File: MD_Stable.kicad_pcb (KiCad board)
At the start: 2 copper layers, 100 x 100 mm, 308 parts, among them J1 Conn_02x04_Counter_Clockwise, J10 Conn_02x06_Odd_Even, J11 Conn_01x08_Pin, J12 Conn_01x05_Socket, J2 XT30_Male, J3 XT60_Male, J4 RE1, J5 RE2, J6 RE3, J7 MO_XT60_Female1, J8 MO_XT60_Female2, J9 MO_XT60_Female3, Q1 MTB7D0N6RJ3, Q10 MTB7D0N6RJ3, Q11 MTB7D0N6RJ3, Q12 MTB7D0N6RJ3, Q2 MTB7D0N6RJ3, Q3 MTB7D0N6RJ3, Q4 MTB7D0N6RJ3, Q5 MTB7D0N6RJ3, Q6 MTB7D0N6RJ3, Q7 MTB7D0N6RJ3, Q8 MTB7D0N6RJ3, Q9 MTB7D0N6RJ3, SW1 SW_Push, SW2 SW_Push, SW3 PWM, SW4 PWM, SW5 PWM, SW6 DIR, SW7 DIR, SW8 DIR, U1 NJM7808SDL1, U10 74AHC1G08W5, U11 74AHC1G08W5, U12 74AHC1G08W5, U13 IRS2302S, U14 IRS2302S, U15 IRS2302S, U16 NE555D, U17 IRS2302S, U18 IRS2302S, U19 IRS2302S, U2 BA05CC0Tに似た何か, U20 74AHC1G08W5, U21 74AHC1G08W5, U22 74AHC1G08W5, U23 UTRS485G-S08-R, U24 UTRS485G-S08-R, U3 STM32G431K8Tx, U4 BA05CC0Tに似た何か, U5 BA033CC0FP, U6 π160M60, U7 74AHC1G04W5, U8 74AHC1G04W5, U9 74AHC1G04W5

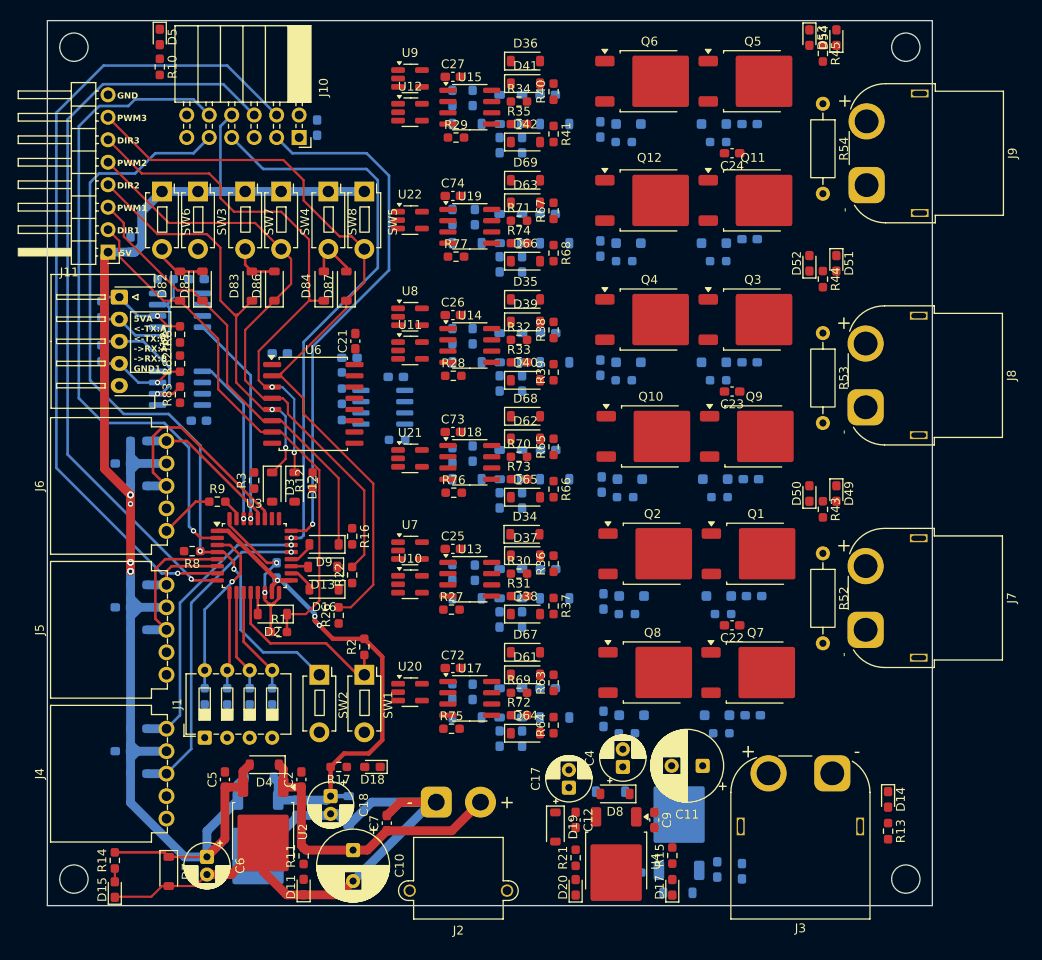
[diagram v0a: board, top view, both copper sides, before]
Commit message: 配線終わり見えてきた
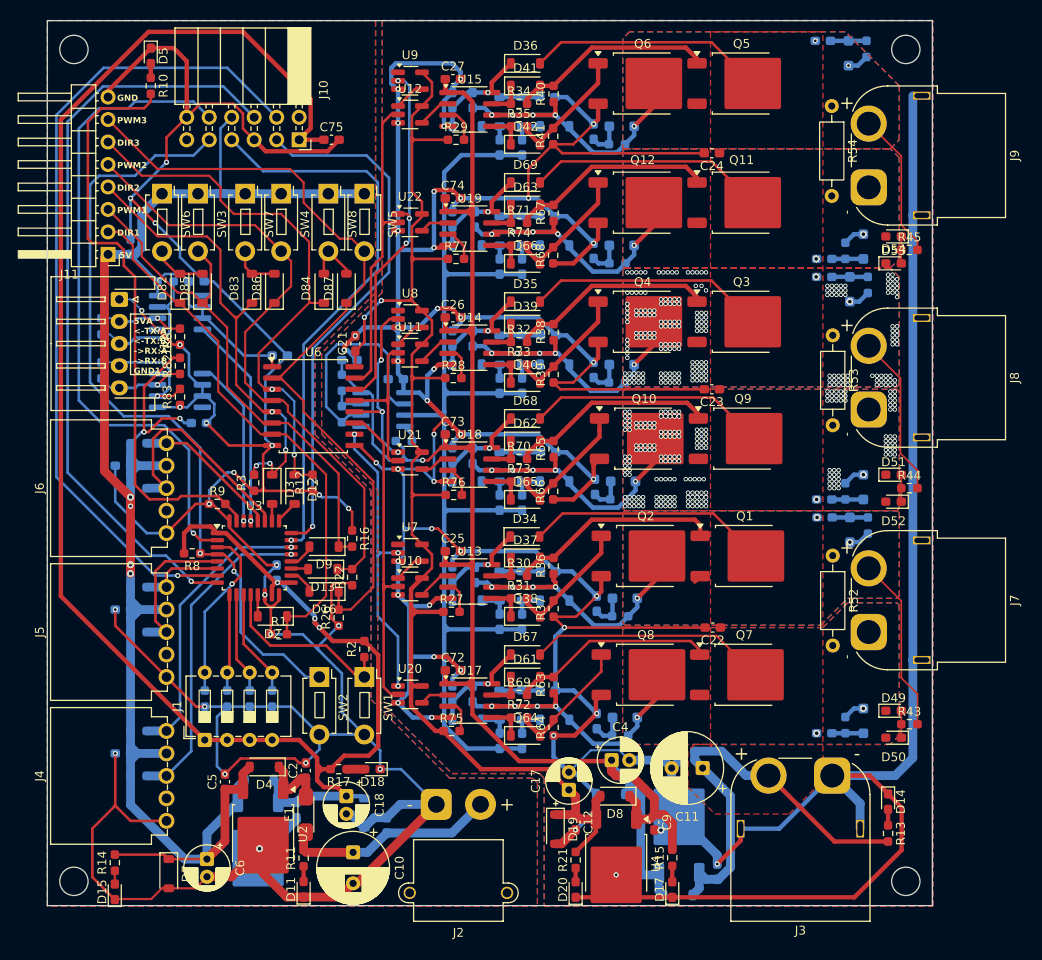
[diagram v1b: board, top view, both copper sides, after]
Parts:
- added F1: Polyfuse, MyLib:PolyFuse_MF-NSMF-series, F.Cu at (130.8, 140.5)
- C7: moved to B.Cu
- C75: moved to F.Cu
- moved D50 29.2 mm to (197.2, 131.8), turned to 180 degrees
- moved D52 28.6 mm to (197.2, 105.2), turned to 180 degrees
- moved D53 27.2 mm to (197.2, 78.2), turned to 0 degrees
- moved R43 26.2 mm to (199.0, 130.3), turned to 0 degrees
- moved R44 25.6 mm to (199.0, 103.6), turned to 0 degrees
- moved D49 25.4 mm to (197.2, 128.8), turned to 0 degrees
- moved D51 24.7 mm to (197.2, 102.1), turned to 0 degrees
- moved R45 24.3 mm to (199.0, 76.7), turned to 0 degrees
- moved D54 23.4 mm to (197.2, 75.2), turned to 180 degrees
- moved R48 20.1 mm to (194.3, 80.7), turned to -90 degrees
- moved R50 19.8 mm to (194.2, 54.0), turned to -90 degrees
- moved R46 19.2 mm to (194.3, 107.9), turned to -90 degrees
- moved D45 17.4 mm to (192.3, 81.2), turned to 90 degrees
- moved D47 17.2 mm to (192.1, 54.5), turned to 90 degrees
- moved D59 16.9 mm to (193.8, 76.3), turned to -90 degrees
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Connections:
- C2 pad 1: +12V -> Net-(D4-K)
- D4 pad 1: +12V -> Net-(D4-K)
- J12 pad 1: Net-(J12-Pin_1) -> GNDD
- J12 pad 5: GNDD -> Net-(J12-Pin_5)
- J3 pad : (no net) -> GND
- J7 pad : (no net) -> GND
- J8 pad : (no net) -> GND
- J9 pad : (no net) -> GND
- R78 pad 1: Net-(J12-Pin_1) -> Net-(J12-Pin_2)
- R78 pad 2: Net-(J12-Pin_2) -> Net-(J12-Pin_3)
- R79 pad 1: Net-(J12-Pin_3) -> Net-(J12-Pin_4)
- R79 pad 2: Net-(J12-Pin_4) -> Net-(J12-Pin_5)
- R80 pad 1: Net-(J12-Pin_2) -> Net-(J12-Pin_3)
- R81 pad 2: Net-(J12-Pin_1) -> Net-(J12-Pin_2)
- R82 pad 1: Net-(J12-Pin_4) -> Net-(J12-Pin_5)
- R83 pad 2: Net-(J12-Pin_3) -> Net-(J12-Pin_4)
- U2 pad 1: +12V -> Net-(D4-K)
- U23 pad 6: Net-(J12-Pin_1) -> Net-(J12-Pin_2)
- U23 pad 7: Net-(J12-Pin_2) -> Net-(J12-Pin_3)
- U24 pad 6: Net-(J12-Pin_3) -> Net-(J12-Pin_4)
- U24 pad 7: Net-(J12-Pin_4) -> Net-(J12-Pin_5)
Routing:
- net GND: track 0.00 -> 596.3 mm, vias 0 -> 43
- net GNDD: track 103.2 -> 388.2 mm, vias 2 -> 24
- net VCC: track 0.00 -> 210.7 mm, vias 0 -> 6
- net +8V: track 0.00 -> 189.4 mm, vias 0 -> 1
- net +5V: track 0.00 -> 154.0 mm, vias 0 -> 2
- net +3V3: track 60.4 -> 208.8 mm
- net 555_Out_A: track 0.00 -> 126.3 mm
- net LED_1: track 2.44 -> 67.7 mm
- net Source_1A: track 0.00 -> 60.0 mm, vias 0 -> 6
- net Source_2A: track 0.00 -> 57.8 mm, vias 0 -> 224
- net Source_3A: track 0.00 -> 56.2 mm, vias 0 -> 6
- net +5VD: track 182.6 -> 227.9 mm, vias 4 -> 8
- net out_DIR3: track 0.00 -> 40.7 mm, vias 0 -> 3
- net Source_1B: track 0.00 -> 40.0 mm, vias 0 -> 6
- net Source_3B: track 0.00 -> 39.8 mm, vias 0 -> 6
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- added copper zone on B.Cu, net GND
- added copper zone on F.Cu, net GND
- added copper zone on B.Cu, net GNDD
- added copper zone on F.Cu, net GNDD
- added copper zone on B.Cu, net Source_1A
- added copper zone on F.Cu, net Source_1A
- added copper zone on B.Cu, net Source_1B
- added copper zone on F.Cu, net Source_1B
- added copper zone on B.Cu, net Source_2A
- added copper zone on F.Cu, net Source_2A
- added copper zone on B.Cu, net Source_2B
- added copper zone on F.Cu, net Source_2B
- added copper zone on B.Cu, net Source_3A
- added copper zone on F.Cu, net Source_3A
- added copper zone on B.Cu, net Source_3B
- added copper zone on F.Cu, net Source_3B
- added copper zone on F.Cu, net VCC

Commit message: MD基板完成
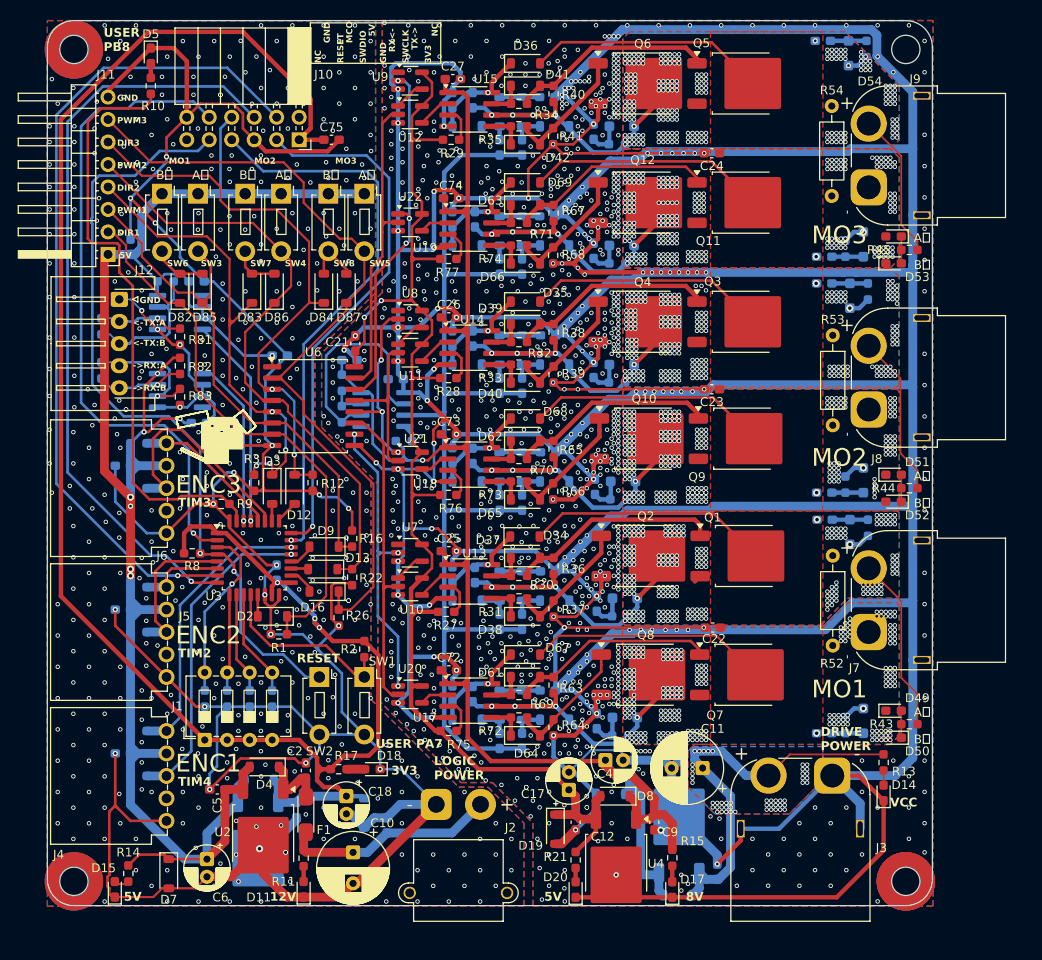
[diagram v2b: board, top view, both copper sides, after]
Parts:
- added G***: LOGO, MyLib:BDCrogidrive_nega, B.Cu at (123.4, 54.6)
- added ref**: val**, MyLib:ROGIKEN, F.Cu at (120.5, 98.3)
- moved R13 8.04 mm to (196.1, 134.6), turned to 90 degrees
- moved R14 1.95 mm to (110.7, 147.2)
- moved C5 1.22 mm to (120.8, 137.7), turned to 180 degrees
- moved D14 1.11 mm to (196.1, 138.1), turned to 90 degrees
- moved R77 0.86 mm to (146.9, 77.7)
- moved C52 0.77 mm to (189.4, 104.1)
- moved D57 0.77 mm to (193.8, 102.7)
- moved R57 0.77 mm to (191.8, 103.2)
- moved C45 0.74 mm to (189.4, 80.5)
- moved R48 0.74 mm to (194.3, 81.4)
- moved D45 0.74 mm to (192.3, 81.9)
- moved C4 0.70 mm to (164.7, 134.4)
- moved R27 0.60 mm to (146.7, 117.6)
- moved R76 0.60 mm to (146.9, 104.4)
- moved R29 0.56 mm to (147.2, 64.3)
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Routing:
- net GND: track 596.3 -> 876.0 mm, vias 43 -> 932
- net +5V: track 154.0 -> 150.8 mm
- net VCC: track 210.7 -> 208.1 mm, vias 6 -> 56
- net GNDD: track 388.2 -> 390.8 mm, vias 24 -> 448
- net DIR2: track 52.8 -> 54.8 mm
- net DIR1: track 61.4 -> 62.7 mm
- net +5VD: track 227.9 -> 226.7 mm
- net +8V: track 189.4 -> 190.5 mm
- net PWM1: track 59.8 -> 60.4 mm
- net Source_2A: vias 224 -> 234
- net Source_3B: vias 6 -> 230
- net Source_3A: vias 6 -> 223
- net Source_2B: vias 216 -> 230
- net Source_1B: vias 6 -> 235
- net Source_1A: vias 6 -> 226
- added copper zone on B.Cu, net VCC
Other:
- outline, holes or cut-outs redrawn
- board text added: "->RX:A"
- board text added: "->RX:B"
- board text added: "12V"
- board text added: "3V3"
- board text added: "8V"
- board text added: "<-TX:A"
- board text added: "<-TX:B"
- board text added: "A相"
- board text added: "B相"
- board text added: "DCMotor Driver Rev3.0 @KayOChef_meme"
- board text added: "DRIVE POWER"
- board text added: "ENC1"
- board text added: "ENC2"
- board text added: "ENC3"
- board text added: "LOGIC POWER"
- board text added: "MCO"
- board text added: "MO1"
- board text added: "MO2"
- board text added: "MO3"
- board text added: "NC"
- board text added: "RESET"
- board text added: "RX<-"
- board text added: "SWCLK"
- board text added: "SWDIO"
- board text added: "TIM2"
- board text added: "TIM3"
- board text added: "TIM4"
- board text added: "TX->"
- board text added: "USER PA7"
- board text added: "USER PB8"
- board text added: "VCC"
- board text removed: "5VA <-TX:A <-TX:B ->RX:A ->RX:B GND1"

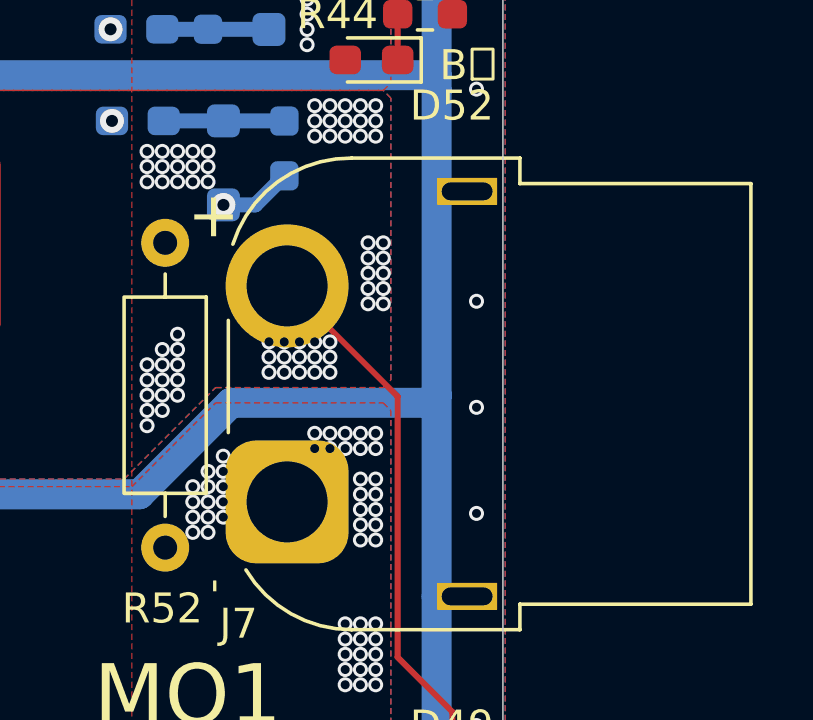
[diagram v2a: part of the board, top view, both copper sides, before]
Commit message: 製造番号位置指定
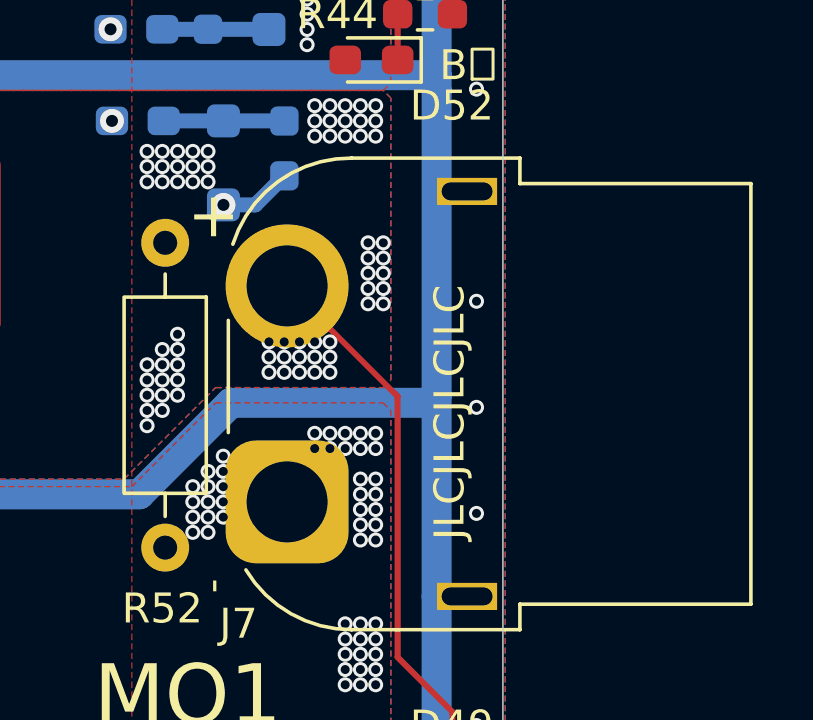
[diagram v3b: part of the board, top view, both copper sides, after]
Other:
- board text added: "JLCJLCJLCJLC"
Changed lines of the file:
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@@
+		)
+	)
+	(gr_text "JLCJLCJLCJLC"
+		(at 200.406 121.158 90)
+		(layer "F.SilkS")
+		(effects
+			(font
+				(size 1 1)
+				(thickness 0.1)
+			)
+			(justify left bottom)
 		)
 	)
